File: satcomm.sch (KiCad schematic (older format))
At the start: 15 parts

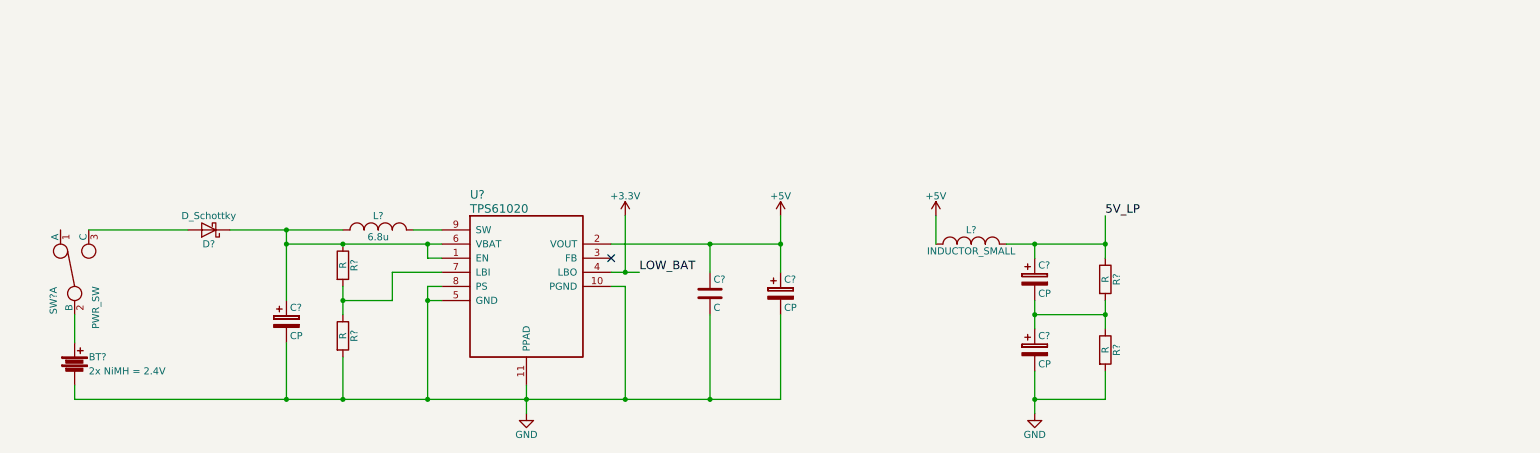
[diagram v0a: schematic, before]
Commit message: circuit extended
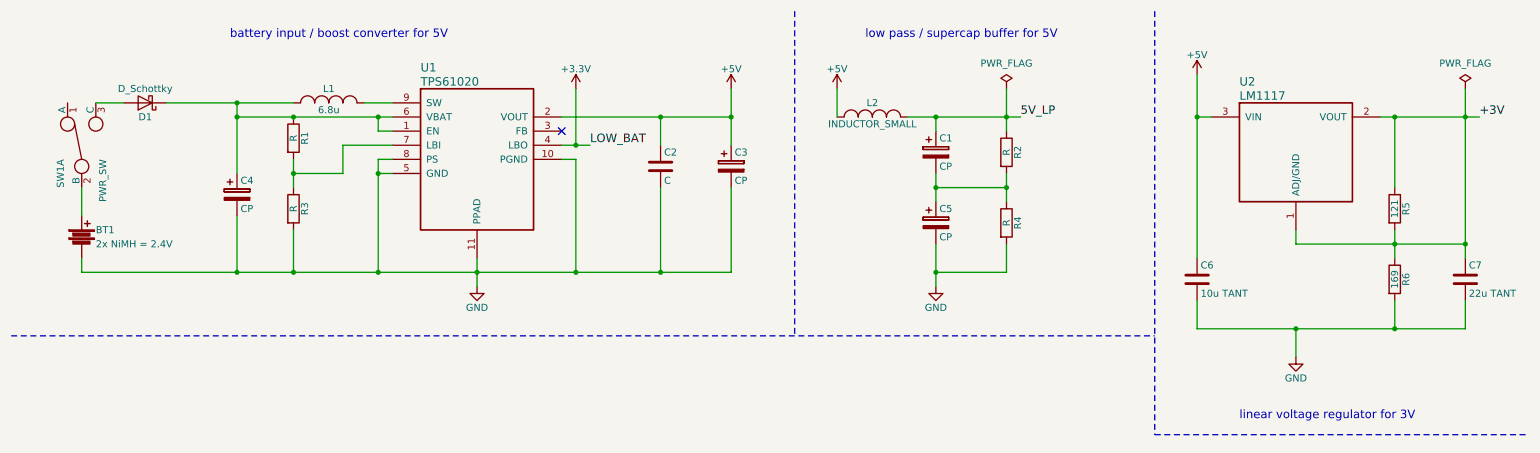
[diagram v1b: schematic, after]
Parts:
- added C6: 10u TANT, symbol C
- added C7: 22u TANT, symbol C
- added R5: 121, symbol R
- added R6: 169, symbol R
- added U2: LM1117, symbol LM1117
- gave numbers to parts that had none: 15
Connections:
- net +5V: now also C6.1, U2.3 (VIN)
- net GND: now also C6.2, C7.2, R6.2
- new net +3V: C7.1, R5.1, R5.2, R6.1, U2.1 (ADJ/GND), U2.2 (VOUT)
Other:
- note added: "battery input / boost converter for 5V"
- note added: "linear voltage regulator for 3V\n"
- note added: "low pass / supercap buffer for 5V"
- moved on the sheet: BT1, C1, C2, C3, C4, C5, D1, L1, L2, R1, R2, R3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
